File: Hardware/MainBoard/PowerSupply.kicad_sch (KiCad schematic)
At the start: 12 parts, among them J5 USB_B_Micro, U3 LD1117ASTR

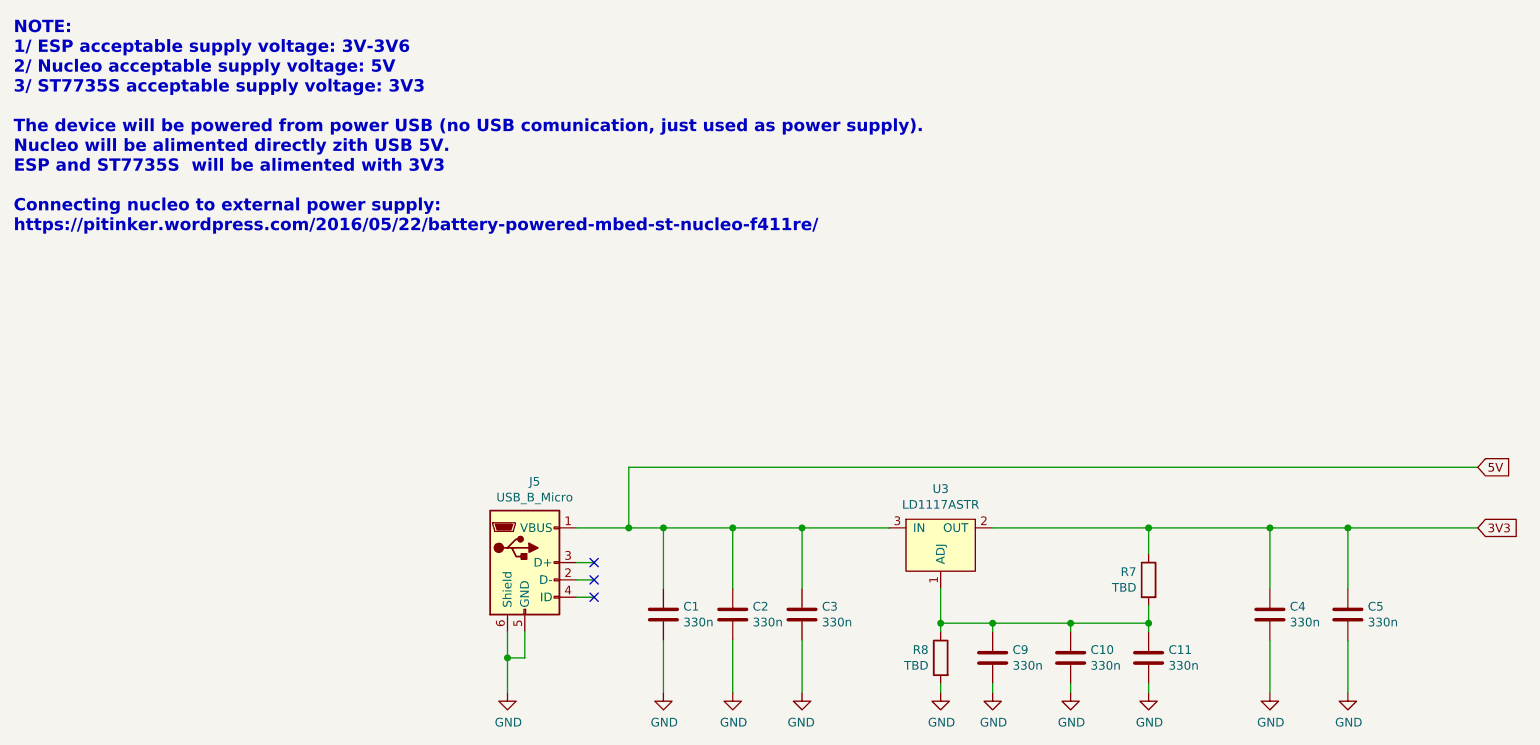
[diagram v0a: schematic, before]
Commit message: pcb draft
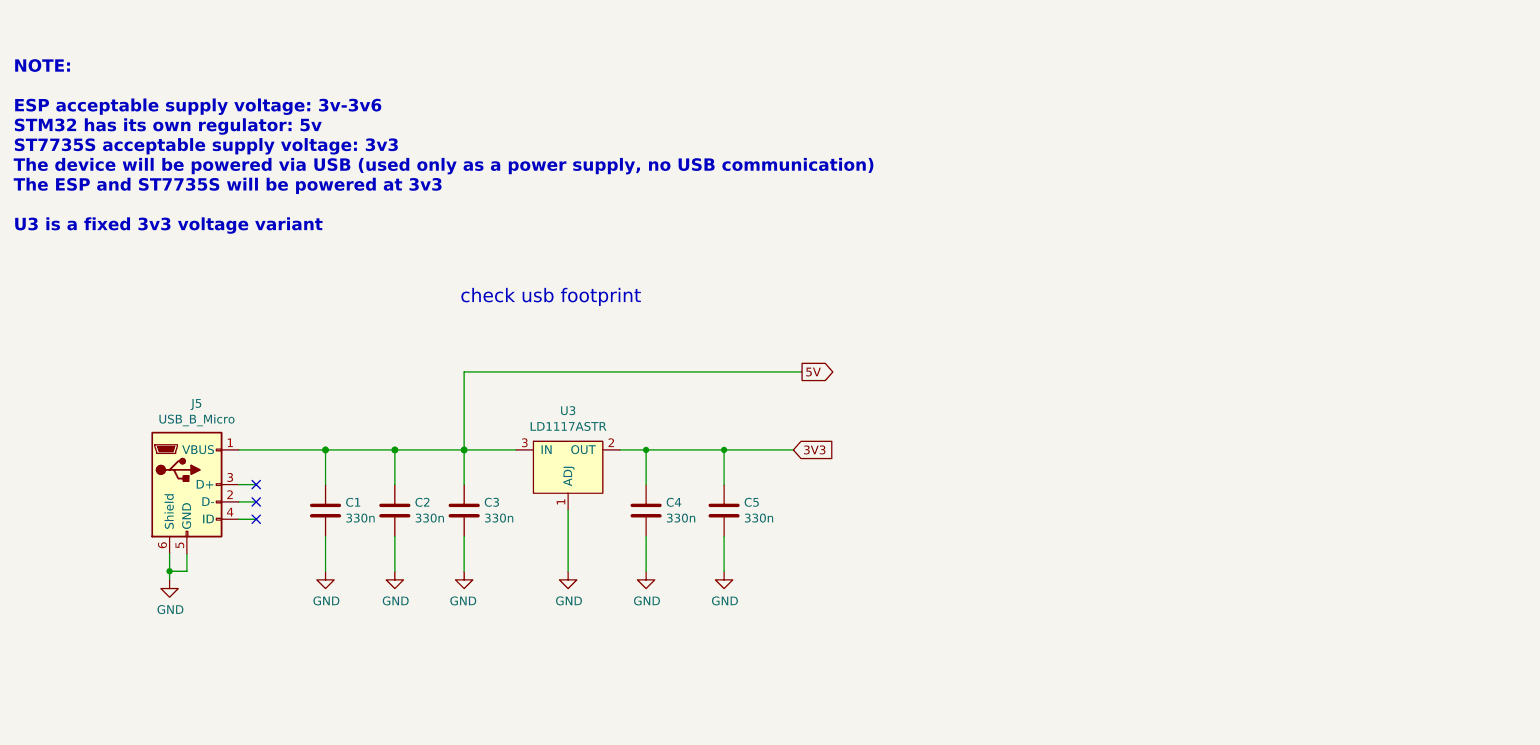
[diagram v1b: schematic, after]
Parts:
- removed C10, C11, C9: 330n, Capacitor_SMD:C_0805_2012Metric, symbol Device:C
- removed R7, R8: TBD, Resistor_SMD:R_0805_2012Metric, symbol Device:R
- U3: symbol Logger:LD1117ASTR -> MainBoard:LD1117ASTR
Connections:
- net GND: now also U3.1 (ADJ)
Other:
- note added: "NOTE: ESP acceptable supply voltage: 3v-3v6 STM32 has its own regulator: 5v ST7735S acceptable supply voltage: 3v3 The device will be powered via USB (used only as a power supply, no USB communication) The ESP and ST7735S will be powered at 3v3 U3 is a fixed 3v3 voltage variant"
- note added: "check usb footprint"
- note removed: "NOTE: 1/ ESP acceptable supply voltage: 3V-3V6 2/ Nucleo acceptable supply voltage: 5V 3/ ST7735S acceptable supply voltage: 3V3 The device will be powered from power USB (no USB comunication, just used as power supply). Nucleo will be alimented directly zith USB 5V. ESP and ST7735S will be alimented with 3V3 Connecting nucleo to external power supply: https://pitinker.wordpress.com/2016/05/22/ba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"
- moved on the sheet: C1, C2, C3, C4, C5, J5, U3
